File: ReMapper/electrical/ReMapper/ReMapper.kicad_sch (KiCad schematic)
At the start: 50 parts, among them J1 QSPI_Debug, J2 USB_IN, J3 USB_IN_Debug, J4 ESP_UART0, J5 USB_OUT, J6 USB_OUT_Debug, U1 ESP32-S3-WROOM-1-N8R8, U2 RP2040, U3 W25Q128JVE, U4 RT6150B-33GQW, U5 W25Q128JVE, Y1 12MHZ

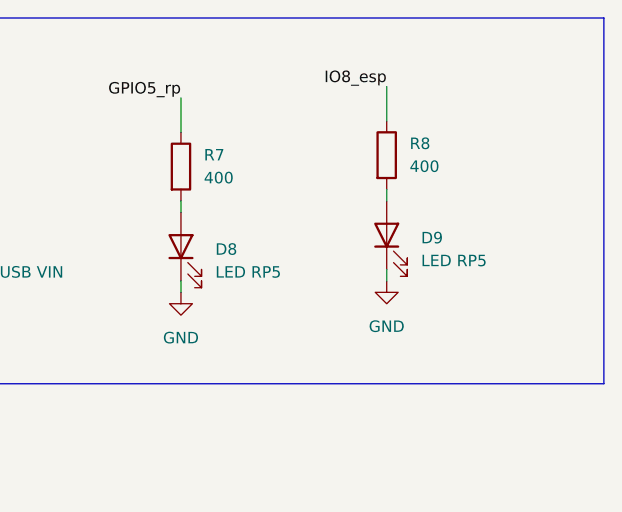
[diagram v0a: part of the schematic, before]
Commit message: started layout
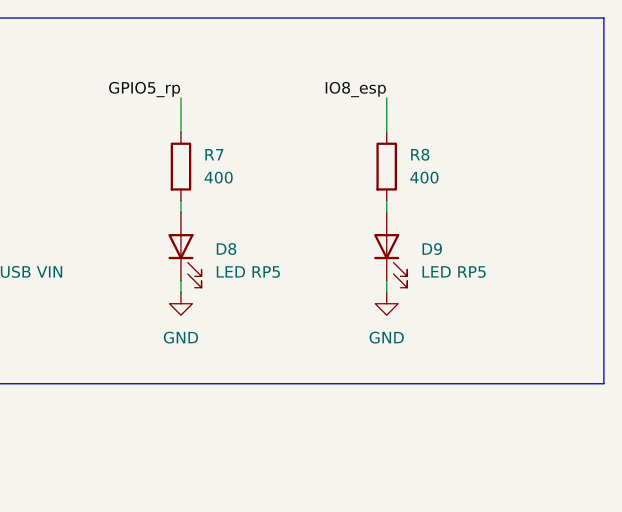
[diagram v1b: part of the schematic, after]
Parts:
- J5: footprint footprints:USBA_Female -> Connector_PinHeader_1.00mm:PinHeader_1x04_P1.00mm_Vertical
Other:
- moved on the sheet: D9, R8
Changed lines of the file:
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@@
 	(wire
 		(pts
-			(xy 382.27 44.45) (xy 382.27 45.72)
+			(xy 382.27 45.72) (xy 382.27 46.99)
 		)
 		(stroke
@@
 	(wire
 		(pts
-			(xy 382.27 24.13) (xy 382.27 27.94)
+			(xy 382.27 25.4) (xy 382.27 29.21)
 		)
 		(stroke
@@
 	(wire
 		(pts
-			(xy 382.27 35.56) (xy 382.27 36.83)
+			(xy 382.27 36.83) (xy 382.27 38.1)
 		)
 		(stroke
@@
 	)
 	(label "IO8_esp"
-		(at 382.27 24.13 180)
+		(at 382.27 25.4 180)
 		(effects
 			(font
@@
 			)
 		)
-		(property "Footprint" "footprints:USBA_Female"
+		(property "Footprint" "Connector_PinHeader_1.00mm:PinHeader_1x04_P1.00mm_Vertical"
 			(at 248.92 76.2 0)
 			(effects
@@
 	(symbol
 		(lib_id "Device:R")
-		(at 382.27 31.75 0)
+		(at 382.27 33.02 0)
 		(unit 1)
 		(exclude_from_sim no)
@@
 		(dnp no)
 		(property "Reference" "R8"
-			(at 384.81 30.4799 0)
+			(at 384.81 31.7499 0)
 			(effects
 				(font
@@
 		)
 		(property "Value" "400"
-			(at 384.81 33.0199 0)
+			(at 384.81 34.2899 0)
 			(effects
 				(font
@@
 		)
 		(property "Footprint" "Resistor_SMD:R_0603_1608Metric"
-			(at 380.492 31.75 90)
+			(at 380.492 33.02 90)
 			(effects
 				(font
@@
 		)
 		(property "Datasheet" "~"
-			(at 382.27 31.75 0)
+			(at 382.27 33.02 0)
 			(effects
 				(font
@@
 		)
 		(property "Description" "Resistor"
-			(at 382.27 31.75 0)
+			(at 382.27 33.02 0)
 			(effects
 				(font
@@
 	(symbol
 		(lib_id "power:GND")
-		(at 382.27 45.72 0)
+		(at 382.27 46.99 0)
 		(unit 1)
 		(exclude_from_sim no)
@@
 		(fields_autoplaced yes)
 		(property "Reference" "#PWR028"
-			(at 382.27 52.07 0)
+			(at 382.27 53.34 0)
 			(effects
 				(font
@@
 		)
 		(property "Value" "GND"
-			(at 382.27 50.8 0)
+			(at 382.27 52.07 0)
 			(effects
 				(font
@@
 		)
 		(property "Footprint" ""
-			(at 382.27 45.72 0)
+			(at 382.27 46.99 0)
 			(effects
 				(font
@@
 		)
 		(property "Datasheet" ""
-			(at 382.27 45.72 0)
+			(at 382.27 46.99 0)
 			(effects
 				(font
@@
 		)
 		(property "Description" "Power symbol creates a global label with name \"GND\" , ground"
-			(at 382.27 45.72 0)
+			(at 382.27 46.99 0)
 			(effects
 				(font
@@
 	(symbol
 		(lib_id "Device:LED")
-		(at 382.27 40.64 90)
+		(at 382.27 41.91 90)
 		(unit 1)
 		(exclude_from_sim no)
@@
 		(fields_autoplaced yes)
 		(property "Reference" "D9"
-			(at 386.08 40.9574 90)
+			(at 386.08 42.2274 90)
 			(effects
 				(font
@@
 		)
 		(property "Value" "LED RP5"
-			(at 386.08 43.4974 90)
+			(at 386.08 44.7674 90)
 			(effects
 				(font
@@
 		)
 		(property "Footprint" "LED_SMD:LED_0603_1608Metric"
-			(at 382.27 40.64 0)
+			(at 382.27 41.91 0)
 			(effects
 				(font
@@
 		)
 		(property "Datasheet" "~"
-			(at 382.27 40.64 0)
+			(at 382.27 41.91 0)
 			(effects
 				(font
@@
 		)
 		(property "Description" "Light emitting diode"
-			(at 382.27 40.64 0)
+			(at 382.27 41.91 0)
 			(effects
 				(font
@@
 		)
 		(property "Sim.Pins" "1=K 2=A"
-			(at 382.27 40.64 0)
+			(at 382.27 41.91 0)
 			(effects
 				(font
